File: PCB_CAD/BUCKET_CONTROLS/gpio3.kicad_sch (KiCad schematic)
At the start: 13 parts, among them U16 MCP23017_I2C4_0x20, U18 MCP23017_I2C4_0x21, U20 MCP23017_I2C4_0x22

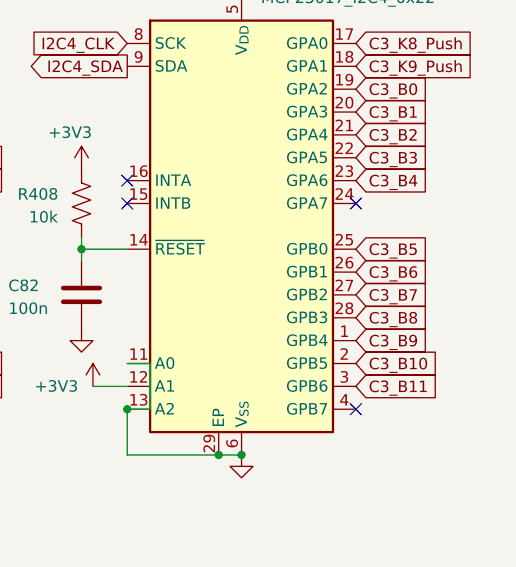
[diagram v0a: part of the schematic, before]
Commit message: pcb routing all day
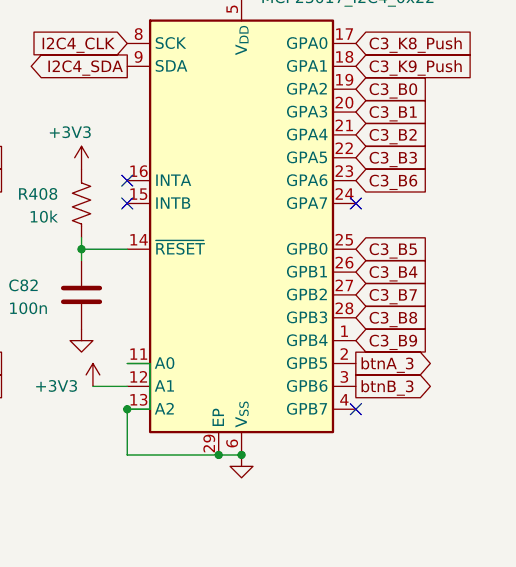
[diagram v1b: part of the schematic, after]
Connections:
- net C3_B4: now also U20.26 (GPB1); no longer U20.23 (GPA6)
- net C3_B6: now also U20.23 (GPA6); no longer U20.26 (GPB1)
- net C3_B10 renamed btnA_3
- net C3_B11 renamed btnB_3
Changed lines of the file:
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@@
 	(global_label "C3_B6"
 		(shape input)
-		(at 196.85 90.17 0)
-		(fields_autoplaced yes)
-		(effects
-			(font
-				(size 1.27 1.27)
-			)
-			(justify left)
-		)
-		(property "Intersheetrefs" "${INTERSHEET_REFS}"
-			(at 205.7618 90.17 0)
+		(at 196.85 80.01 0)
+		(fields_autoplaced yes)
+		(effects
+			(font
+				(size 1.27 1.27)
+			)
+			(justify left)
+		)
+		(property "Intersheetrefs" "${INTERSHEET_REFS}"
+			(at 205.7618 80.01 0)
 			(hide yes)
 			(show_name no)
@@
 		)
 	)
-	(global_label "C3_B10"
-		(shape input)
-		(at 196.85 100.33 0)
-		(fields_autoplaced yes)
-		(effects
-			(font
-				(size 1.27 1.27)
-			)
-			(justify left)
-		)
-		(property "Intersheetrefs" "${INTERSHEET_REFS}"
-			(at 206.9713 100.33 0)
-			(hide yes)
-			(show_name no)
-			(do_not_autoplace no)
-			(effects
-				(font
-					(size 1.27 1.27)
-				)
-				(justify left)
-			)
-		)
-	)
 	(global_label "C3_K1_Push"
 		(shape input)
@@
 		(property "Intersheetrefs" "${INTERSHEET_REFS}"
 			(at 103.8594 87.63 0)
+			(hide yes)
+			(show_name no)
+			(do_not_autoplace no)
+			(effects
+				(font
+					(size 1.27 1.27)
+				)
+				(justify left)
+			)
+		)
+	)
+	(global_label "btnB_3"
+		(shape output)
+		(at 196.85 102.87 0)
+		(fields_autoplaced yes)
+		(effects
+			(font
+				(size 1.27 1.27)
+				(color 255 255 255 1)
+			)
+			(justify left)
+		)
+		(property "Intersheetrefs" "${INTERSHEET_REFS}"
+			(at 206.306 102.87 0)
 			(hide yes)
 			(show_name no)
@@
 	(global_label "C3_B4"
 		(shape input)
-		(at 196.85 80.01 0)
-		(fields_autoplaced yes)
-		(effects
-			(font
-				(size 1.27 1.27)
-			)
-			(justify left)
-		)
-		(property "Intersheetrefs" "${INTERSHEET_REFS}"
-			(at 205.7618 80.01 0)
+		(at 196.85 90.17 0)
+		(fields_autoplaced yes)
+		(effects
+			(font
+				(size 1.27 1.27)
+			)
+			(justify left)
+		)
+		(property "Intersheetrefs" "${INTERSHEET_REFS}"
+			(at 205.7618 90.17 0)
 			(hide yes)
 			(show_name no)
@@
 		)
 	)
-	(global_label "C3_B11"
-		(shape input)
-		(at 196.85 102.87 0)
-		(fields_autoplaced yes)
-		(effects
-			(font
-				(size 1.27 1.27)
-			)
-			(justify left)
-		)
-		(property "Intersheetrefs" "${INTERSHEET_REFS}"
-			(at 206.9713 102.87 0)
-			(hide yes)
-			(show_name no)
+	(global_label "btnA_3"
+		(shape output)
+		(at 196.85 100.33 0)
+		(fields_autoplaced yes)
+		(effects
+			(font
+				(size 1.27 1.27)
+				(color 255 255 255 1)
+			)
+			(justify left)
+		)
+		(property "Intersheetrefs" "${INTERSHEET_REFS}"
+			(at 206.1246 100.33 0)
+			(hide yes)
+			(show_name no)
